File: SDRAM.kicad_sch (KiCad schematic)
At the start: 34 parts, among them U8 IS42S32400F-6TLI

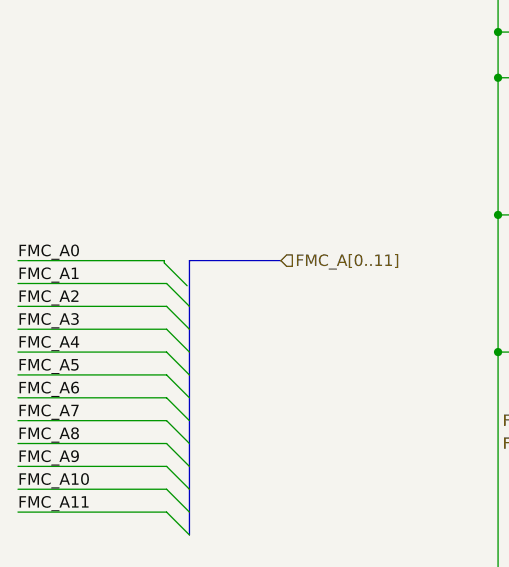
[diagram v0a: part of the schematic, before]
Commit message: started the layout
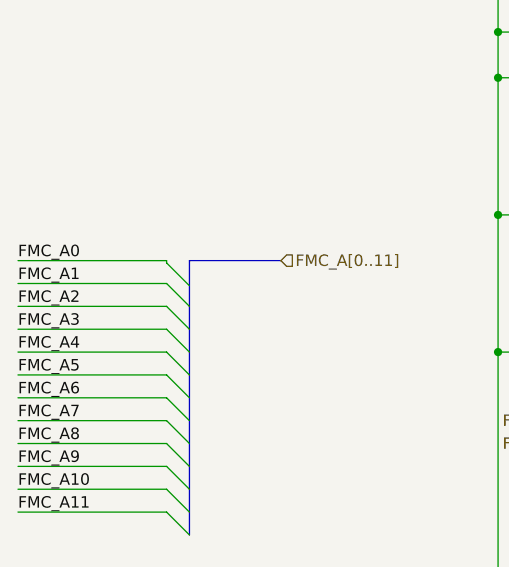
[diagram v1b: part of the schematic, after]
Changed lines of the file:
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@@
 	)
 	(bus_entry
-		(at 42.926 73.914)
+		(at 43.18 73.914)
 		(size -2.54 -2.54)
 		(stroke
@@
 		)
 	)
+	(bus
+		(pts
+			(xy 43.18 73.914) (xy 43.18 76.2)
+		)
+		(stroke
+			(width 0)
+			(type default)
+		)
+	)
 	(wire
 		(pts
@@
 	(bus
 		(pts
-			(xy 43.18 71.12) (xy 43.18 76.2)
+			(xy 43.18 71.12) (xy 43.18 73.914)
 		)
 		(stroke
@@
 	(wire
 		(pts
-			(xy 24.13 71.12) (xy 40.386 71.12)
+			(xy 24.13 71.12) (xy 40.64 71.12)
 		)
 		(stroke
@@
 	(wire
 		(pts
-			(xy 40.386 71.374) (xy 40.386 71.12)
-		)
-		(stroke
+			(xy 40.64 71.374) (xy 40.64 71.12)
+		)
+		(stroke
